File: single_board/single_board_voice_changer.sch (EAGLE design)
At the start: 26 parts, among them U1 ATMEGA328P_PDIP

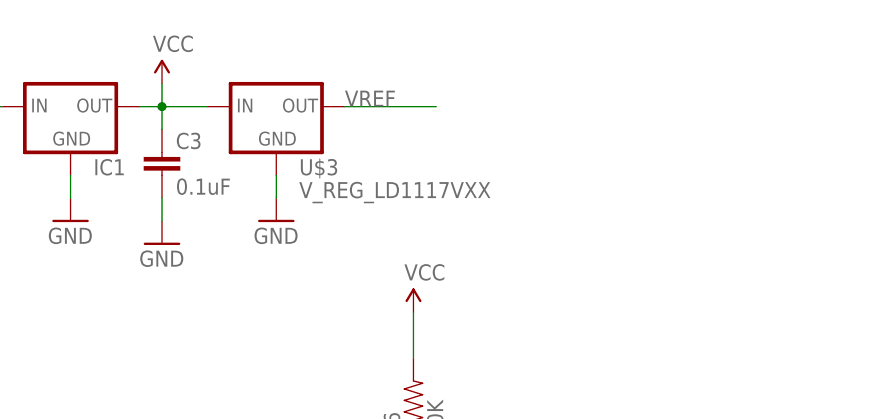
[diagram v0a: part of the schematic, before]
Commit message: working on single board version
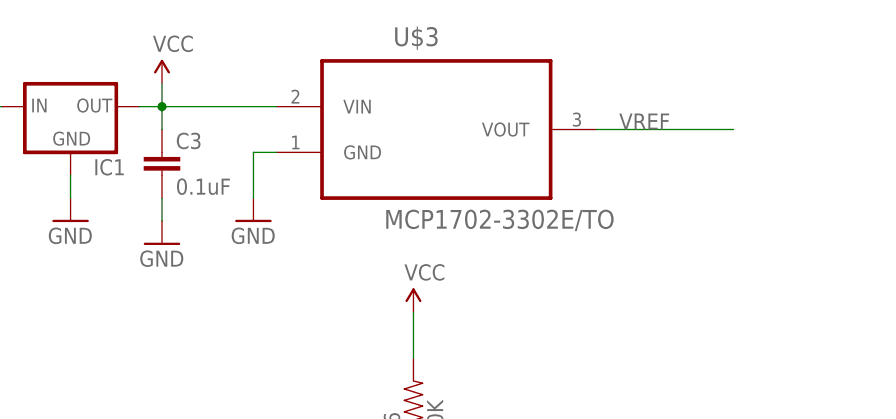
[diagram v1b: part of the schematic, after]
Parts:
- U$3: value V_REG_LD1117VXX -> MCP1702-3302E/TO; device SparkFun-PowerIC:V_REG_LD1117VXX -> Microchip_By_element14_Batch_1:MCP1702-3302E/TO
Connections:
- net VCC: now also U$3.VIN; no longer U$3.IN
- net VREF: now also U$3.VOUT; no longer U$3.OUT
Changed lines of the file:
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@@
 <part name="GND10" library="SparkFun-Aesthetics" deviceset="GND" device=""/>
 <part name="SUPPLY1" library="SparkFun-Aesthetics" deviceset="VCC" device=""/>
-<part name="U$3" library="SparkFun-PowerIC" deviceset="V_REG_LD1117VXX" device=""/>
 <part name="SUPPLY2" library="SparkFun-Aesthetics" deviceset="VCC" device=""/>
 <part name="GND11" library="SparkFun-Aesthetics" deviceset="GND" device=""/>
@@
 <part name="INPUT3" library="SparkFun-Connectors" deviceset="M03" device="PTH"/>
 <part name="INPUT4" library="SparkFun-Connectors" deviceset="M03" device="PTH"/>
+<part name="U$3" library="Microchip_By_element14_Batch_1" deviceset="MCP1702-3302E/TO" device=""/>
 </parts>
 <sheets>
@@
 <instance part="GND10" gate="1" x="-27.94" y="91.44"/>
 <instance part="SUPPLY1" gate="G$1" x="-17.78" y="106.68"/>
-<instance part="U$3" gate="G$1" x="-5.08" y="104.14"/>
 <instance part="SUPPLY2" gate="G$1" x="25.4" y="63.5"/>
-<instance part="GND11" gate="1" x="-5.08" y="91.44"/>
+<instance part="GND11" gate="1" x="-7.62" y="91.44"/>
 <instance part="GND12" gate="1" x="-17.78" y="88.9"/>
 <instance part="C3" gate="G$1" x="-17.78" y="96.52"/>
@@
 <instance part="INPUT3" gate="G$1" x="48.26" y="-30.48"/>
 <instance part="INPUT4" gate="G$1" x="73.66" y="-30.48"/>
+<instance part="U$3" gate="A" x="12.7" y="104.14"/>
 </instances>
 <busses>
@@
 </segment>
 <segment>
-<pinref part="GND11" gate="1" pin="GND"/>
-<pinref part="U$3" gate="G$1" pin="GND"/>
-<wire x1="-5.08" y1="93.98" x2="-5.08" y2="96.52" width="0.1524" layer="91"/>
-</segment>
-<segment>
 <pinref part="GND12" gate="1" pin="GND"/>
 <pinref part="C3" gate="G$1" pin="2"/>
@@
 <wire x1="81.28" y1="-33.02" x2="91.44" y2="-33.02" width="0.1524" layer="91"/>
 <label x="81.28" y="-33.02" size="1.778" layer="95"/>
+</segment>
+<segment>
+<pinref part="U$3" gate="A" pin="GND"/>
+<wire x1="-5.08" y1="99.06" x2="-7.62" y2="99.06" width="0.1524" layer="91"/>
+<pinref part="GND11" gate="1" pin="GND"/>
+<wire x1="-7.62" y1="99.06" x2="-7.62" y2="93.98" width="0.1524" layer="91"/>
 </segment>
 </net>
@@
 <wire x1="-17.78" y1="104.14" x2="-17.78" y2="106.68" width="0.1524" layer="91"/>
 <junction x="-17.78" y="104.14"/>
-<pinref part="U$3" gate="G$1" pin="IN"/>
-<wire x1="-17.78" y1="104.14" x2="-12.7" y2="104.14" width="0.1524" layer="91"/>
 <pinref part="C3" gate="G$1" pin="1"/>
 <wire x1="-17.78" y1="101.6" x2="-17.78" y2="104.14" width="0.1524" layer="91"/>
+<pinref part="U$3" gate="A" pin="VIN"/>
+<wire x1="-5.08" y1="104.14" x2="-17.78" y2="104.14" width="0.1524" layer="91"/>
 </segment>
 <segment>
@@
 </segment>
 <segment>
-<pinref part="U$3" gate="G$1" pin="OUT"/>
-<wire x1="2.54" y1="104.14" x2="12.7" y2="104.14" width="0.1524" layer="91"/>
-<label x="2.54" y="104.14" size="1.778" layer="95"/>
-</segment>
-<segment>
 <pinref part="INPUT1" gate="G$1" pin="3"/>
 <wire x1="5.08" y1="-27.94" x2="15.24" y2="-27.94" width="0.1524" layer="91"/>
@@
 <label x="81.28" y="-27.94" size="1.778" layer="95"/>
 </segment>
-</net>
+<segment>
+<pinref part="U$3" gate="A" pin="VOUT"/>
+<wire x1="30.48" y1="101.6" x2="45.72" y2="101.6" width="0.1524" layer="91"/>
+<label x="33.02" y="101.6" size="1.778" layer="95"/>
+</segment>
+</net>
